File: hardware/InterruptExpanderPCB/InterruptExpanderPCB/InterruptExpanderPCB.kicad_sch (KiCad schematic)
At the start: 4 parts, among them J1 Power, J2 Digital/PWM, J3 Analog, J4 Digital/PWM

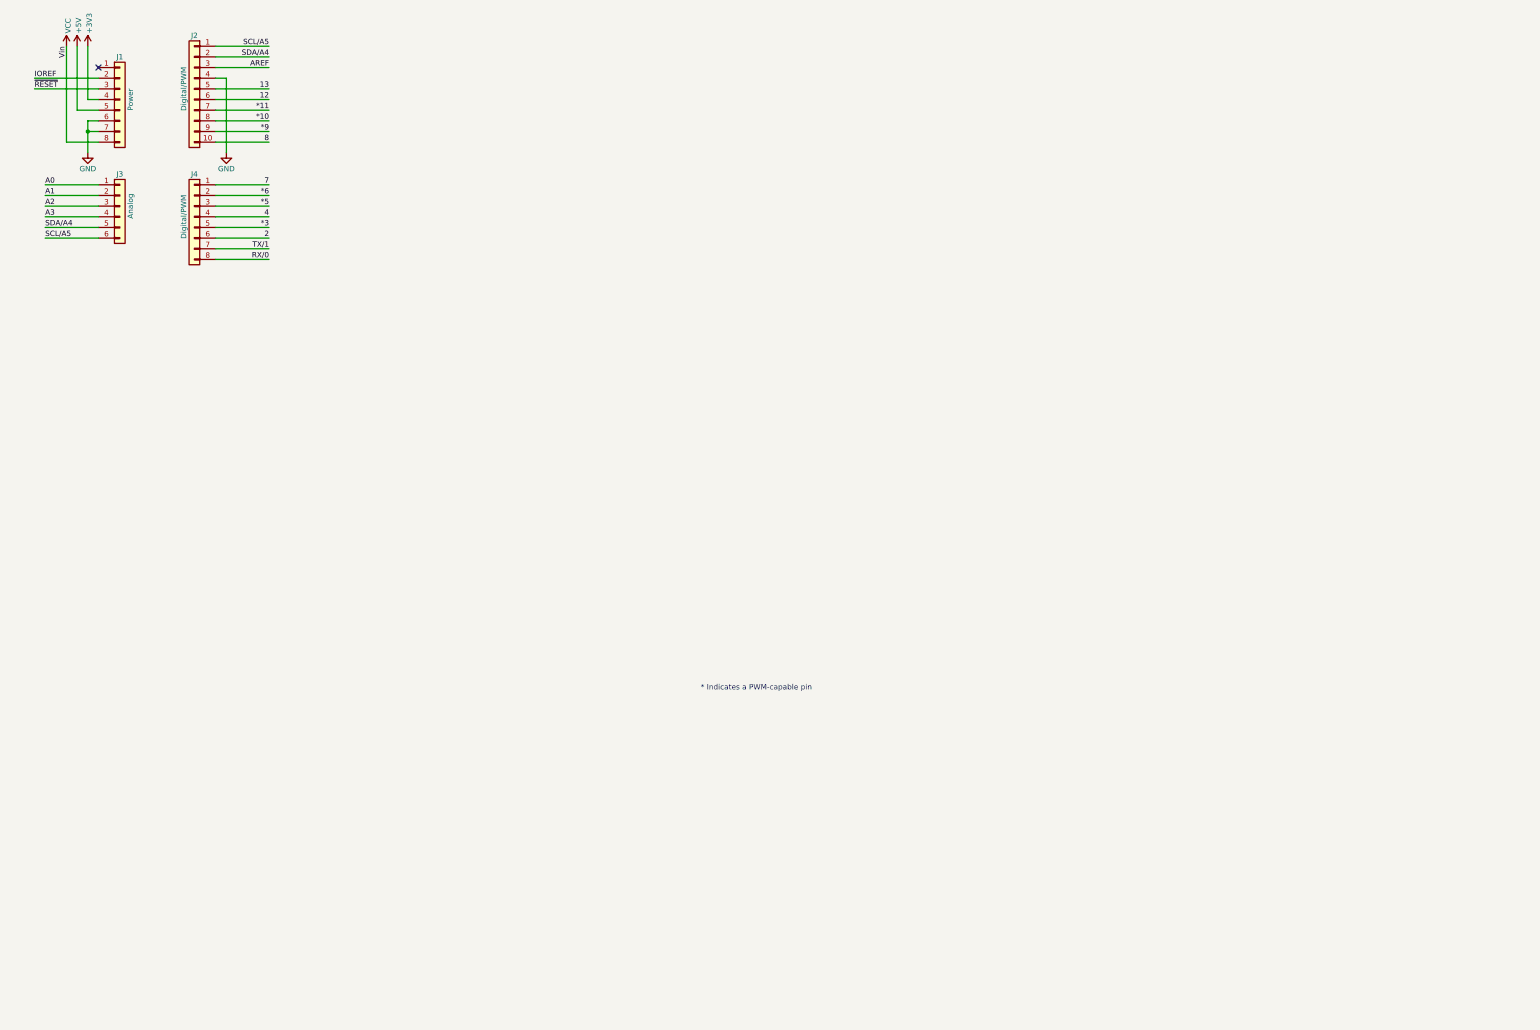
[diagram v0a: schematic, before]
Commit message: working on tests
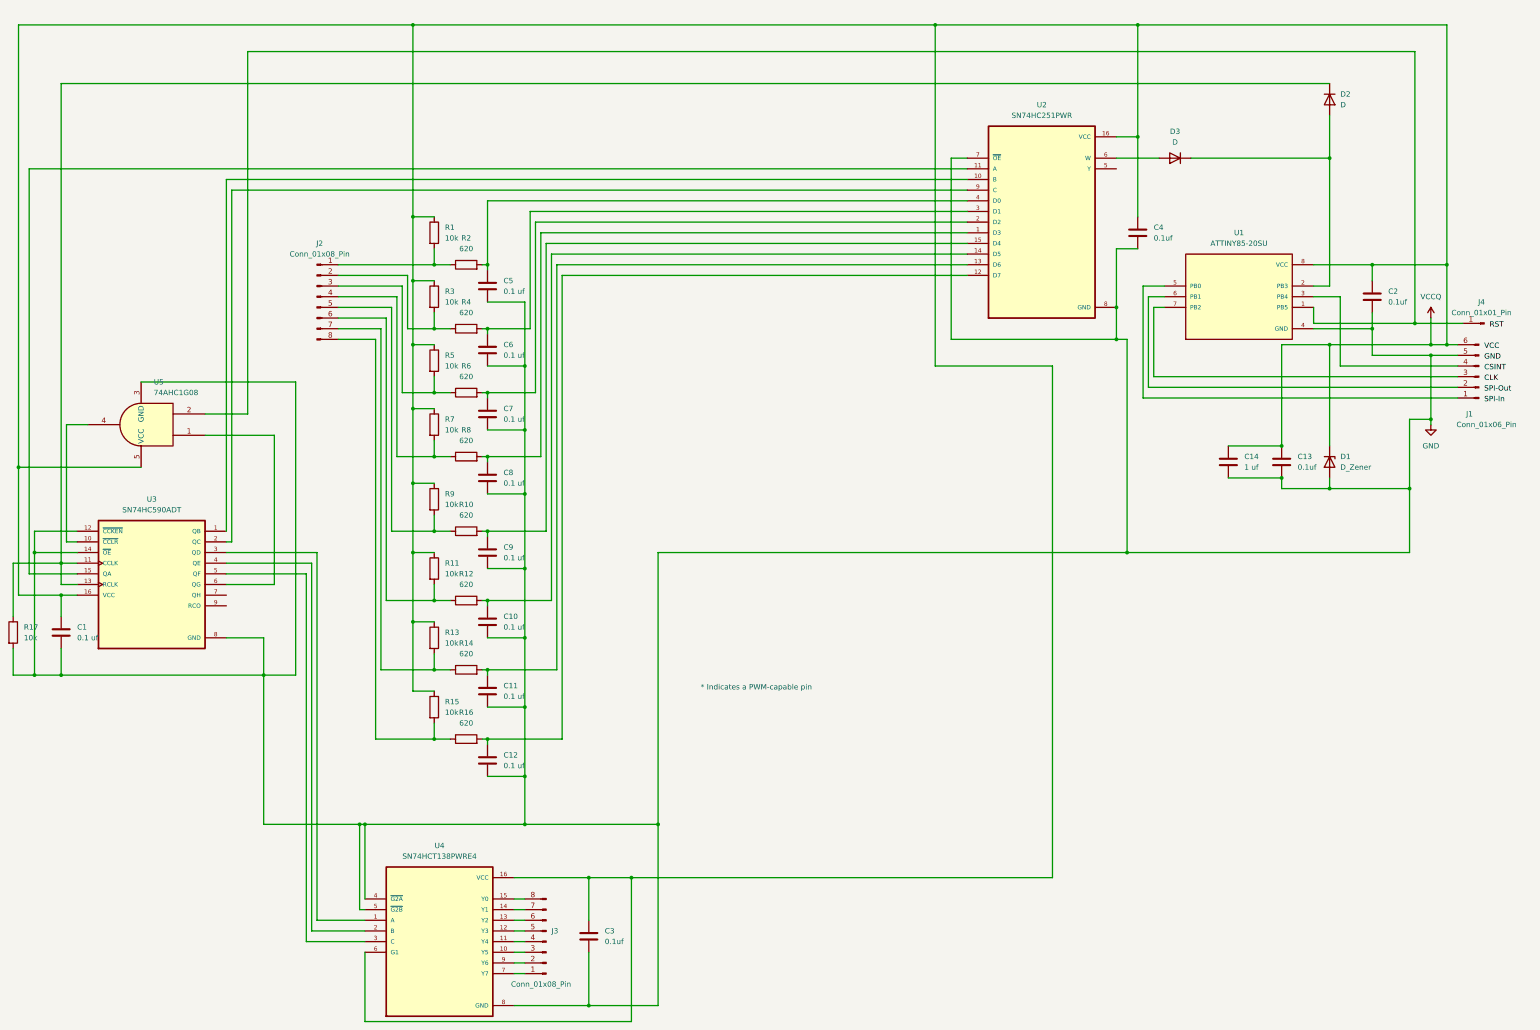
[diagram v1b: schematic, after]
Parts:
- removed J1: Power, Connector_PinSocket_2.54mm:PinSocket_1x08_P2.54mm_Vertical, symbol Connector_Generic:Conn_01x08
- removed J2: Digital/PWM, Connector_PinSocket_2.54mm:PinSocket_1x10_P2.54mm_Vertical, symbol Connector_Generic:Conn_01x10
- removed J3: Analog, Connector_PinSocket_2.54mm:PinSocket_1x06_P2.54mm_Vertical, symbol Connector_Generic:Conn_01x06
- removed J4: Digital/PWM, Connector_PinSocket_2.54mm:PinSocket_1x08_P2.54mm_Vertical, symbol Connector_Generic:Conn_01x08
- added C1, C10, C11, C12, C5, C6, C7, C8, C9: 0.1 uf, Capacitor_SMD:C_0402_1005Metric, symbol Device:C
- added C13, C2, C3, C4: 0.1uf, Capacitor_SMD:C_0402_1005Metric, symbol Device:C
- added C14: 1 uf, Capacitor_SMD:C_0603_1608Metric, symbol Device:C
- added D1: D_Zener, Diode_SMD:D_SOD-123, symbol Device:D_Zener
- added D2, D3: D, InterrupterLibrary:RF01128, symbol Device:D
- added J1: Conn_01x06_Pin, Connector_PinHeader_2.00mm:PinHeader_1x06_P2.00mm_Vertical, symbol Connector:Conn_01x06_Pin
- added J2, J3: Conn_01x08_Pin, Connector_PinHeader_2.00mm:PinHeader_1x08_P2.00mm_Vertical, symbol Connector:Conn_01x08_Pin
- added J4: Conn_01x01_Pin, symbol Connector:Conn_01x01_Pin
- added R1, R11, R13, R15, R17, R3, R5, R7, R9: 10k, Capacitor_SMD:C_0402_1005Metric, symbol Device:R
- added R10, R12, R14, R16, R2, R4, R6, R8: 620, Capacitor_SMD:C_0402_1005Metric, symbol Device:R
- added U1: ATTINY85-20SU, InterrupterLibrary:SOIC127P798X216-8N, symbol ATTINY85-20SU:ATTINY85-20SU
- added U2: SN74HC251PWR, InterrupterLibrary:SOP65P640X120-16N, symbol SN74HC251PWR:SN74HC251PWR
- added U3: SN74HC590ADT, InterrupterLibrary:SOIC127P600X175-16N, symbol SN74HC590ADT:SN74HC590ADT
- added U4: SN74HCT138PWRE4, InterrupterLibrary:SOP65P640X120-16N, symbol SN74HCT138PWRE4:SN74HCT138PWRE4
- added U5: 74AHC1G08, Package_TO_SOT_SMD:SOT-353_SC-70-5_Handsoldering, symbol 74xGxx:74AHC1G08
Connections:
- net GND: now also C1.2, C10.2, C11.2, C12.2, C13.2, C14.2, C2.2, C3.2, C4.2, C5.2, C6.2, C7.2, C8.2, C9.2, D1.2 (A), J1.5 (Pin_5), R17.2, U1.4 (GND), U2.7 (~{OE}), U2.8 (GND), U3.12 (~{CCKEN}), U3.14 (~{OE}), U3.8 (GND), U4.4 (~{G2A}), U4.5 (~{G2B}), U4.8 (GND), U5.3 (GND)
- new net: C5.1, R2.2, U2.4 (D0)
- new net: J2.2 (Pin_2), R3.2, R4.1
- new net: C7.1, R6.2, U2.2 (D2)
- new net: U2.10 (B), U3.1 (QB)
- new net: U3.10 (~{CCLR}), U5.4
- new net: D2.1 (K), R17.1, U3.11 (CCLK), U3.13 (RCLK)
- new net: U2.11 (A), U3.15 (QA)
- new net: U2.9 (C), U3.2 (QC)
- new net: U3.3 (QD), U4.1 (A)
- new net: U3.4 (QE), U4.2 (B)
- new net: U3.5 (QF), U4.3 (C)
- new net: U3.6 (QG), U5.1
- new net: J2.6 (Pin_6), R11.2, R12.1
- new net: J4.1 (Pin_1), U1.1 (PB5), U5.2
- new net: J1.1 (Pin_1), U1.5 (PB0)
- new net: J1.2 (Pin_2), U1.6 (PB1)
- new net: J1.3 (Pin_3), U1.7 (PB2)
- new net: J1.4 (Pin_4), U1.3 (PB4)
- new net: C8.1, R8.2, U2.1 (D3)
- new net: C12.1, R16.2, U2.12 (D7)
- new net: C11.1, R14.2, U2.13 (D6)
- new net: C10.1, R12.2, U2.14 (D5)
- new net: C9.1, R10.2, U2.15 (D4)
- new net: C6.1, R4.2, U2.3 (D1)
- new net: D3.2 (A), U2.6 (W)
- new net: D2.2 (A), D3.1 (K), U1.2 (PB3)
- new net: J2.3 (Pin_3), R5.2, R6.1
- new net: J2.8 (Pin_8), R15.2, R16.1
- new net: J2.5 (Pin_5), R10.1, R9.2
- new net: J2.7 (Pin_7), R13.2, R14.1
- new net: J2.1 (Pin_1), R1.2, R2.1
- new net: J2.4 (Pin_4), R7.2, R8.1
- new net: J3.1 (Pin_1), U4.7 (Y7)
- new net: J3.2 (Pin_2), U4.9 (Y6)
- new net: J3.3 (Pin_3), U4.10 (Y5)
- new net: J3.4 (Pin_4), U4.11 (Y4)
- new net: J3.5 (Pin_5), U4.12 (Y3)
- new net: J3.6 (Pin_6), U4.13 (Y2)
- new net: J3.7 (Pin_7), U4.14 (Y1)
- new net: J3.8 (Pin_8), U4.15 (Y0)
- new net VCCQ: C1.1, C13.1, C14.1, C2.1, C3.1, C4.1, D1.1 (K), J1.6 (Pin_6), R1.1, R11.1, R13.1, R15.1, R3.1, R5.1, R7.1, R9.1, U1.8 (VCC), U2.16 (VCC), U3.16 (VCC), U4.16 (VCC), U4.6 (G1), U5.5 (VCC)
- no-connect marks 1 -> 0
